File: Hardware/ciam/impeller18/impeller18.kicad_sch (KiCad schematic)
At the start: 36 parts, among them J1 BH1,27-10-G, J2 PLS-6, SW1 SW_RESET, SW2 MSS-12D16, SW3 MSS-12D16, U1 STM32F427ZGTx, Y1 X322516MLB4SI, Y2 KSE-7K32768KDY2400A3

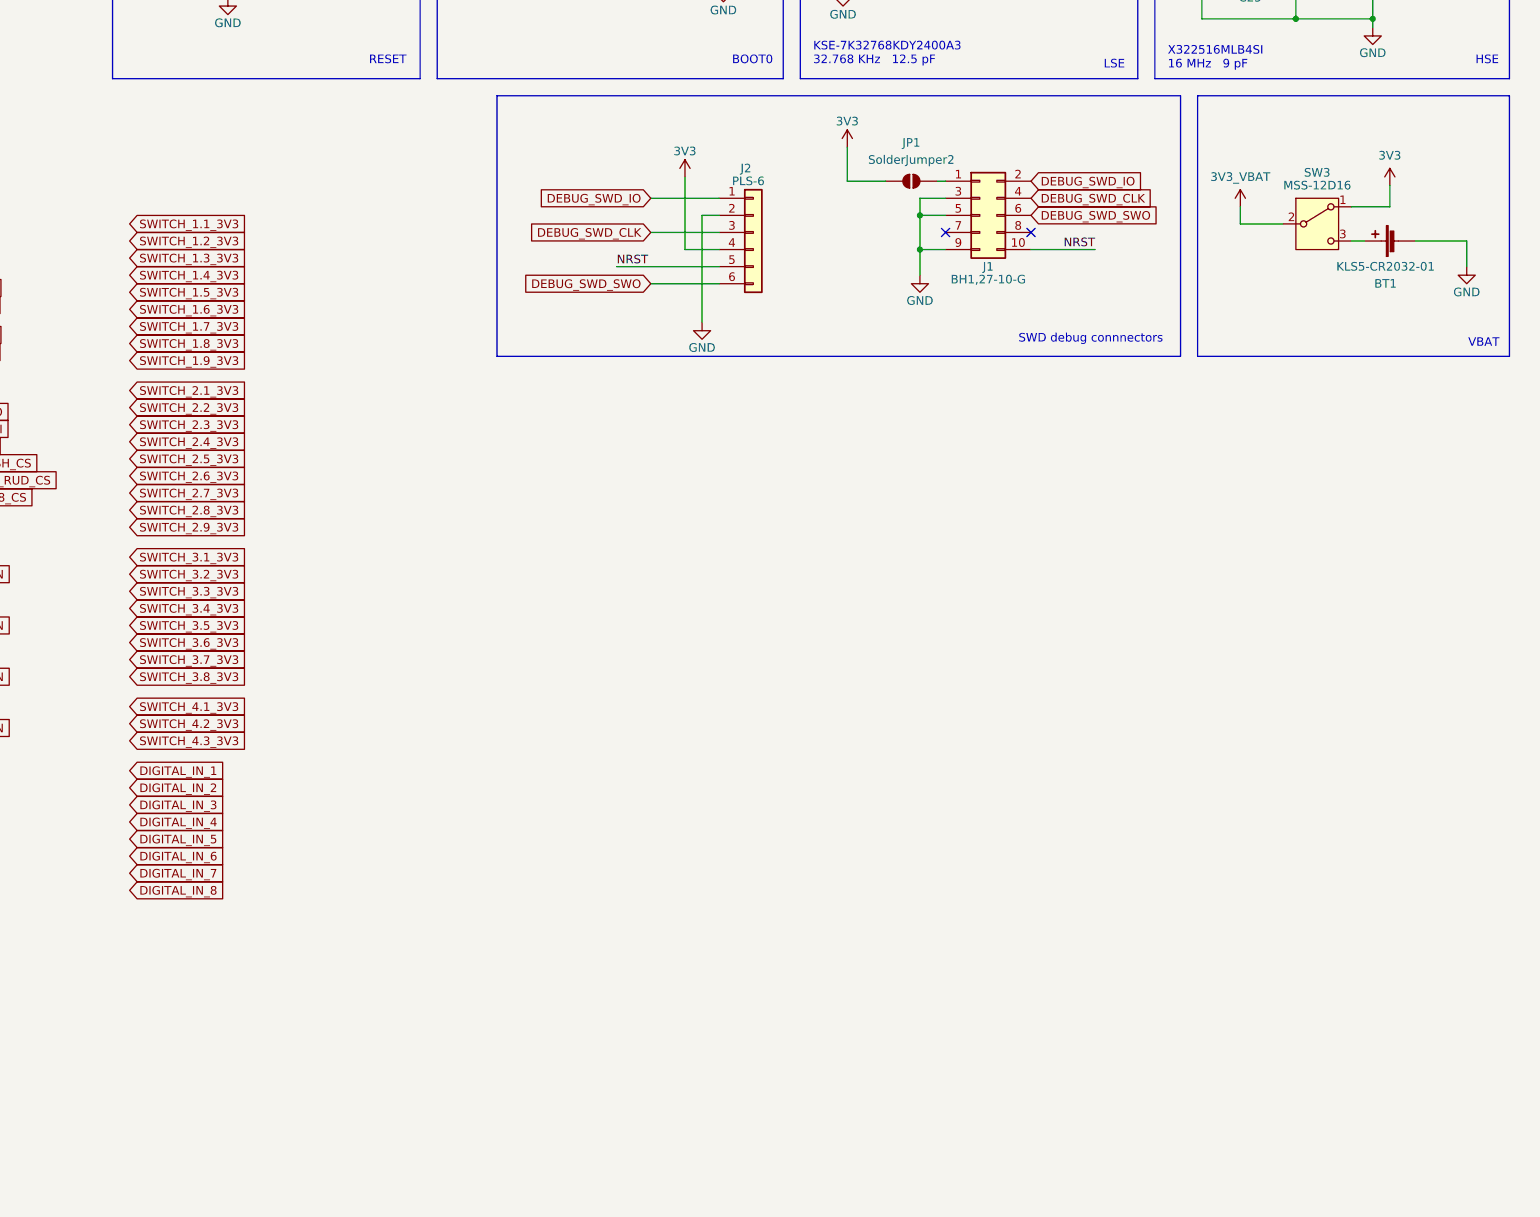
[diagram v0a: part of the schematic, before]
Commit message: updated schematics
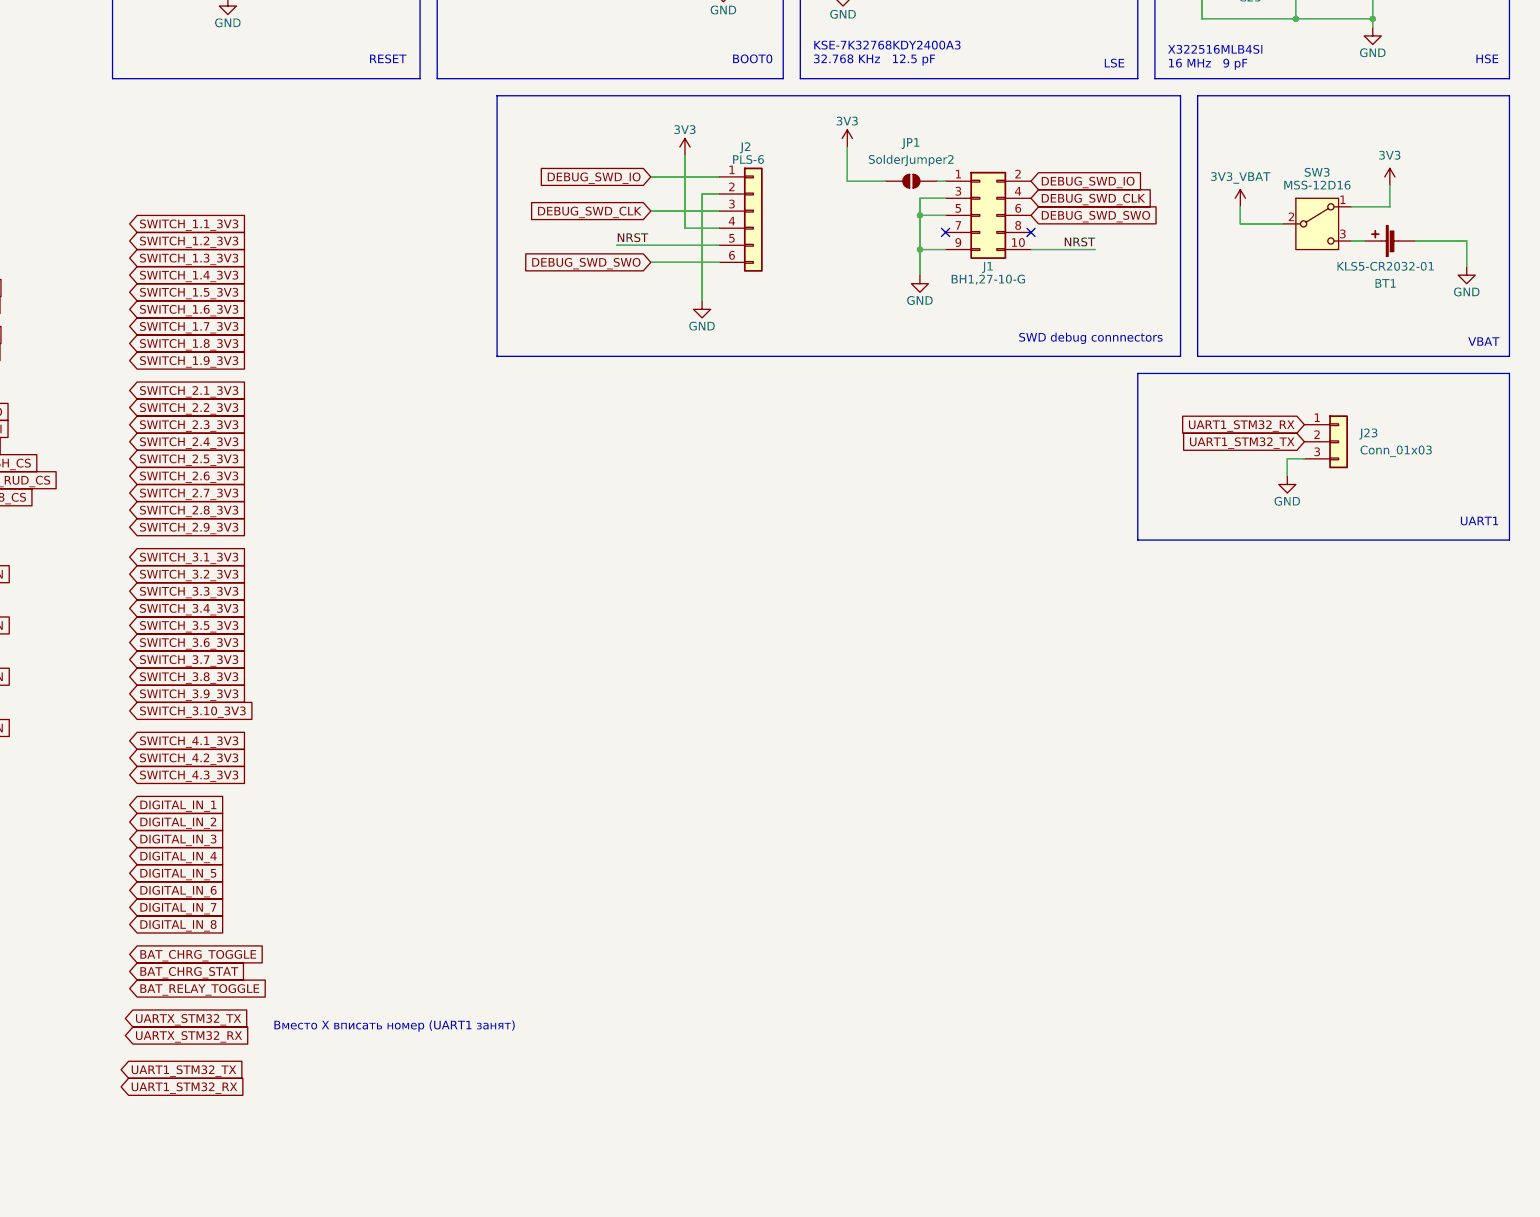
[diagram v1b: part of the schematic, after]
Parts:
- added J23: Conn_01x03, symbol Connector_Generic:Conn_01x03
- BT1: Ссылка https://www.chipdip.ru/product/bh-642 -> (none); Цена 16 -> (none); Человекопонятное название Разъем для плоской батарейки 3В -> (none)
- C22, C24: Ссылка https://www.chipdip.ru/product/grm1885c2a150j -> (none); Цена 6 -> (none); Человекопонятное название Конденсатор 15пФ -> (none)
- Y2: Ссылка https://www.chipdip.ru/product0/8022143960 -> (none); Человекопонятное название Кристаллический резонатор 32КГц -> (none)
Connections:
- net GND: now also J23.3 (Pin_3)
- new net UART1_STM32_RX: J23.1 (Pin_1)
- new net UART1_STM32_TX: J23.2 (Pin_2)
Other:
- note added: "UART1"
- note added: "Вместо X вписать номер (UART1 занят)"
- moved on the sheet: J2
